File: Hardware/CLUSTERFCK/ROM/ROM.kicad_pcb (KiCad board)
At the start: 2 copper layers, 142 x 60.3 mm, 11 parts, among them J1 Conn_02x20_Counter_Clockwise, J2 Conn_02x20_Counter_Clockwise, J4 Conn_02x08_Counter_Clockwise, J6 Conn_02x06_Counter_Clockwise, SW3 SW_DIP_x02, U30 28c64, U31 28c64

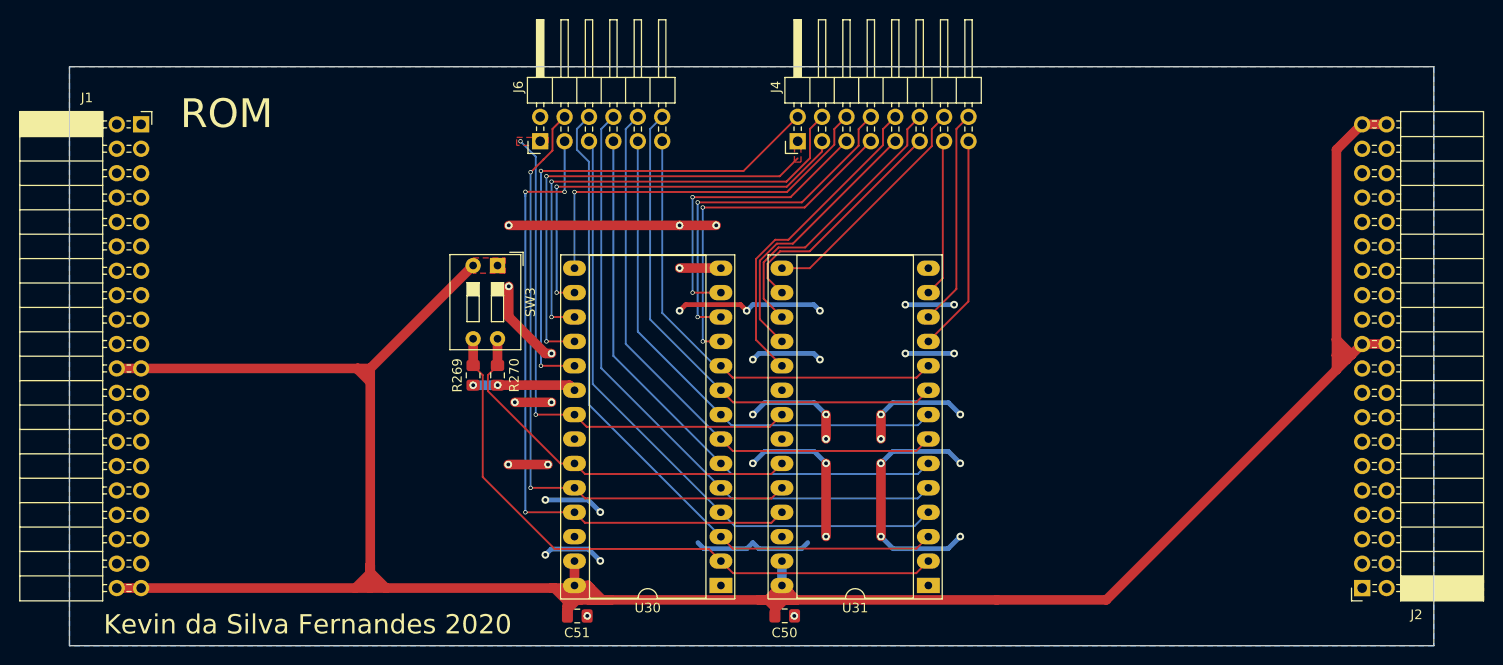
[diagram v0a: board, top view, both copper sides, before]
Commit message: 0049 | 1h | review ROM
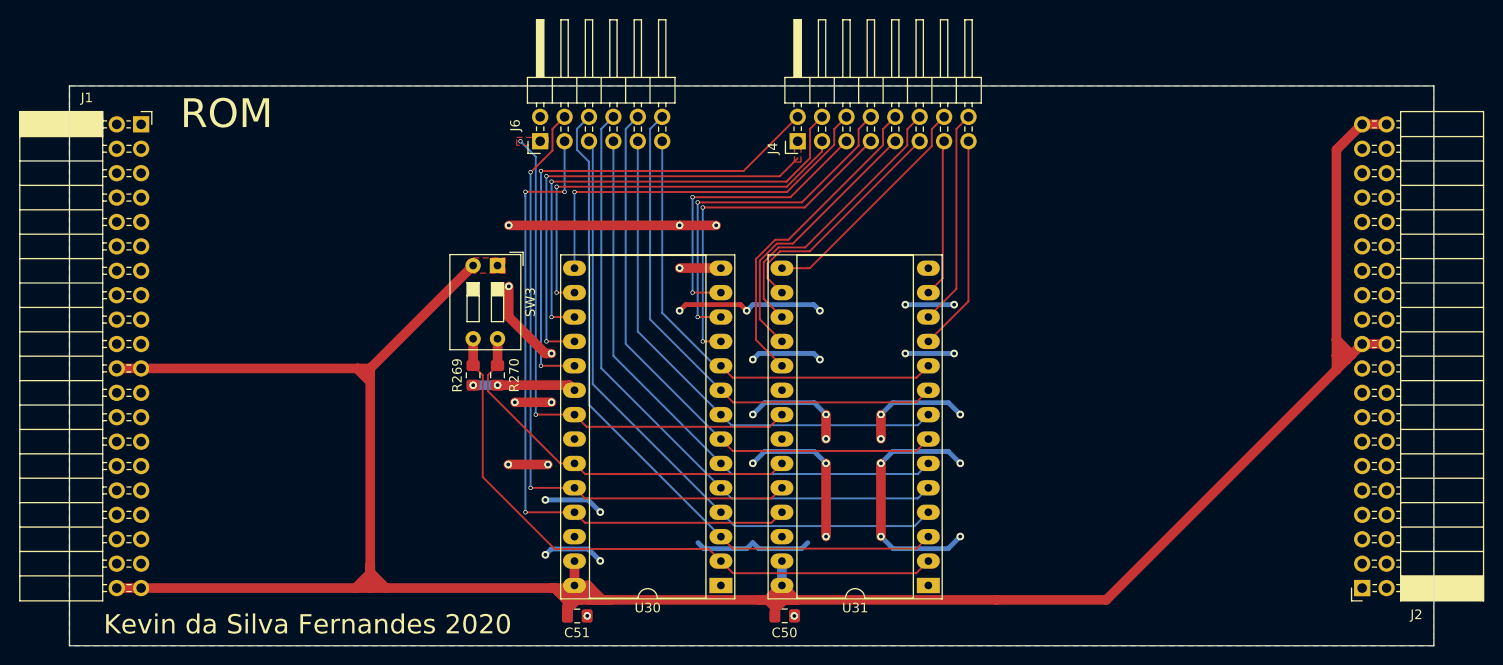
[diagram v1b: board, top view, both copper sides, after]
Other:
- board size 142 x 60.3 mm -> 142 x 58.3 mm
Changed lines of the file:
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@@
     (descr "Through hole angled pin header, 2x08, 2.54mm pitch, 6mm pin length, double rows")
     (tags "Through hole angled pin header THT 2x08 2.54mm double row")
-    (fp_text reference "J4" (at 5.655 -2.27 90) (layer "F.SilkS")
+    (fp_text reference "J4" (at -0.744 -2.587 90) (layer "F.SilkS")
       (effects (font (size 1 1) (thickness 0.15)))
     )
@@
     (descr "Through hole angled pin header, 2x06, 2.54mm pitch, 6mm pin length, double rows")
     (tags "Through hole angled pin header THT 2x06 2.54mm double row")
-    (fp_text reference "J6" (at 5.655 -2.27 90) (layer "F.SilkS")
+    (fp_text reference "J6" (at 1.656 -2.59 90) (layer "F.SilkS")
       (effects (font (size 1 1) (thickness 0.15)))
     )
@@
     (effects (font (size 3 3) (thickness 0.5)))
   )
-  (gr_line (start 142 0) (end 142 60.26) (layer "Edge.Cuts") (width 0.05))
-  (gr_line (start 0 0) (end 0 60.26) (layer "Edge.Cuts") (width 0.05))
+  (gr_line (start 142 2) (end 142 60.26) (layer "Edge.Cuts") (width 0.05))
+  (gr_line (start 0 2) (end 0 60.26) (layer "Edge.Cuts") (width 0.05))
   (gr_line (start 0 60.26) (end 142 60.26) (layer "Edge.Cuts") (width 0.05))
-  (gr_line (start 0 0) (end 142 0) (layer "Edge.Cuts") (width 0.05))
+  (gr_line (start 0 2) (end 142 2) (layer "Edge.Cuts") (width 0.05))
   (segment (start 43.54999 32.09751) (end 43.54999 33.75999) (width 0.2) (layer "F.Cu") (net 31))
   (segment (start 44.55 31.0975) (end 43.54999 32.09751) (width 0.2) (layer "F.Cu") (net 31))
@@
     (polygon
       (pts
-        (xy 142 60.26) (xy 0 60.26) (xy 0 0) (xy 142 0)
+        (xy 142 60.26) (xy 0 60.26) (xy 0 2) (xy 142 2)
       )
     )
